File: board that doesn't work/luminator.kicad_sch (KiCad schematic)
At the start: 37 parts, among them J1 Board #1 Large Connector, J2 Board #3 Large Connector, J3 Board #1 Small Connector, J4 Board #3 Small Connector, J5 Board #2 Large Connector, J6 Board #4 Large Connector, J7 Board #2 Small Connector, J8 Board #4 Small Connector, U1 Temperature_Module, U10 MPQ6628, U11 MPQ6628, U12 MPQ6628, U13 MPQ6628, U14 MPQ6628, U15 MPQ6628, U2 ESP-01, U3 RTC_Module, U4 MPQ6628, U5 MPQ6628, U6 MPQ6628, U7 MPQ6628, U8 MPQ6628, U9 MPQ6628

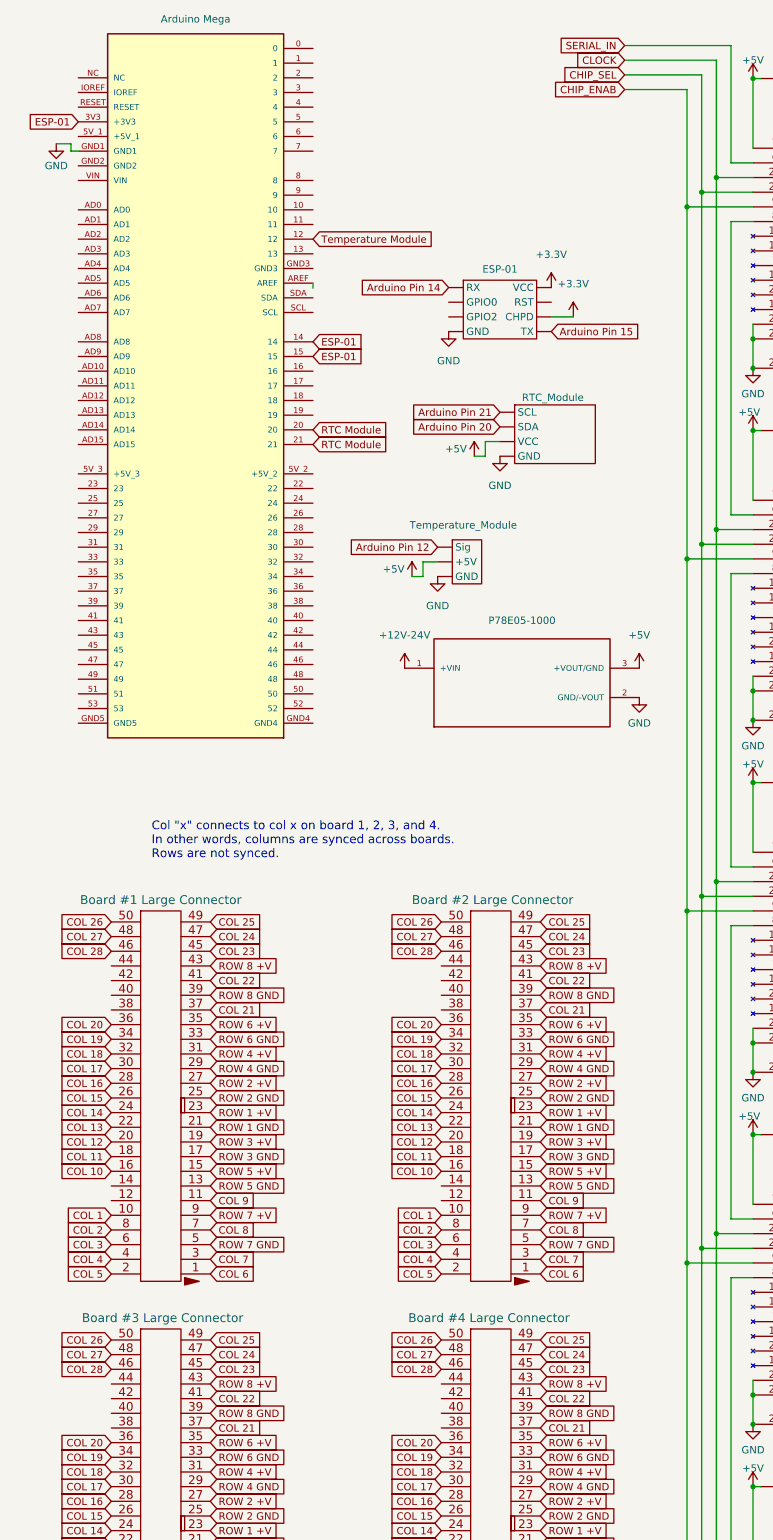
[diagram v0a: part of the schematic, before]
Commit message: asd
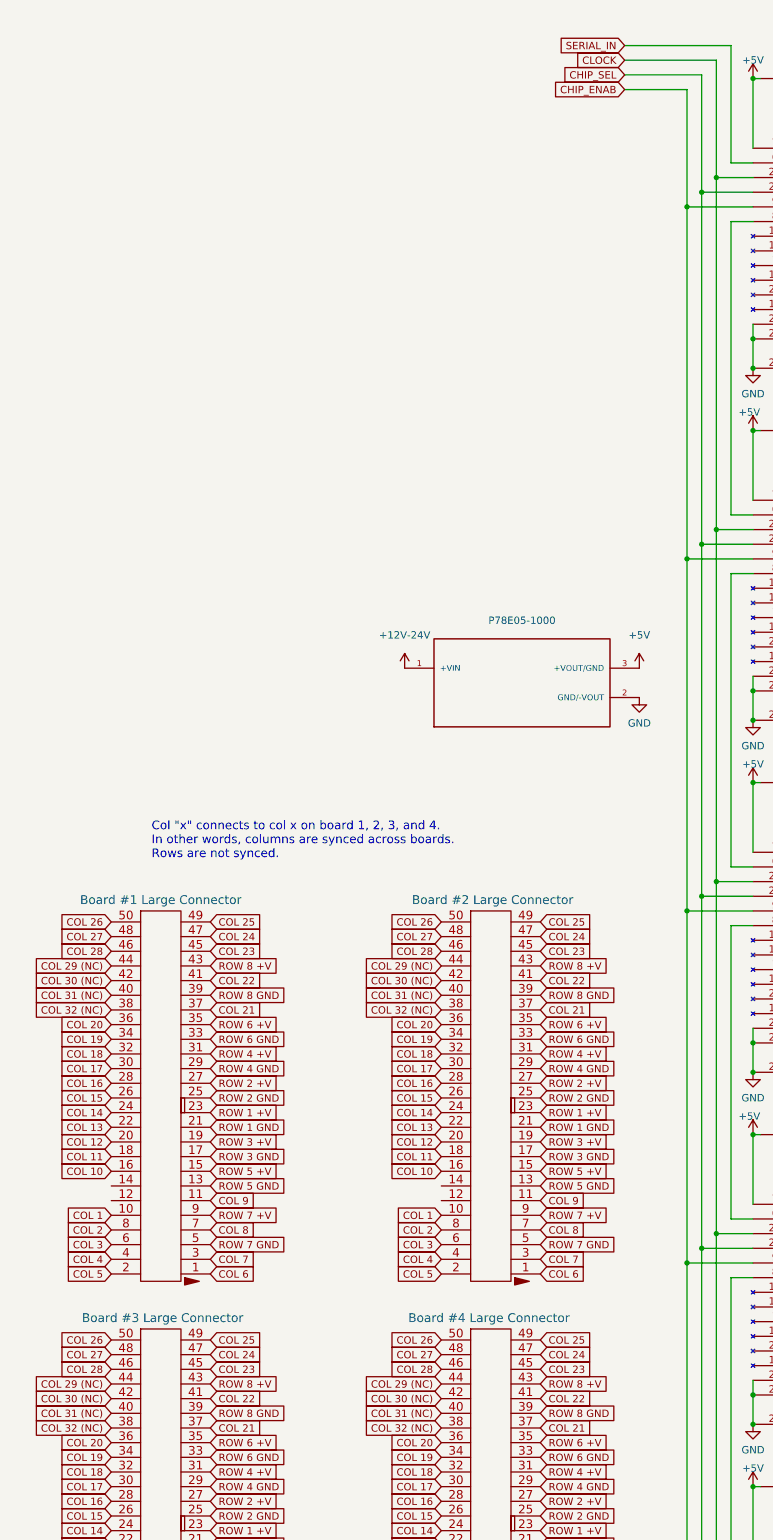
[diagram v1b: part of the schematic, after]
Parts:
- removed A1: Arduino Mega, ARDUINO_A000067, symbol Luminator:Arduino Mega
- removed U1: Temperature_Module, symbol Luminator:Temperature_Module
- removed U2: ESP-01, symbol Luminator:ESP-01
- removed U3: RTC_Module, symbol Luminator:RTC_Module
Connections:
- net COL 29 (NC): now also J1.44, J2.44, J5.44, J6.44
- net COL 30 (NC): now also J1.42, J2.42, J5.42, J6.42
- net COL 31 (NC): now also J1.40, J2.40, J5.40, J6.40
- net COL 32 (NC): now also J1.38, J2.38, J5.38, J6.38
